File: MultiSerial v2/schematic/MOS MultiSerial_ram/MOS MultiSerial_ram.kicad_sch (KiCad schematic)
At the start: 36 parts, among them J10 ., J11 ., J12 Conn_01x01, J13 Conn_01x04, J14 Conn_01x02, J24 Conn_01x01, J6 Conn_01x04, J7 Conn_02x04_Odd_Even, J8 ., J9 Conn_01x01, U1 6551, U10 74AHC1G08, U2 74HC14, U3 65C52, U4 MC6850, U5 IS63WV1288DBLL-10xLI, U6 74LVC253, U7 74LVC595, U8 74AHC1G14

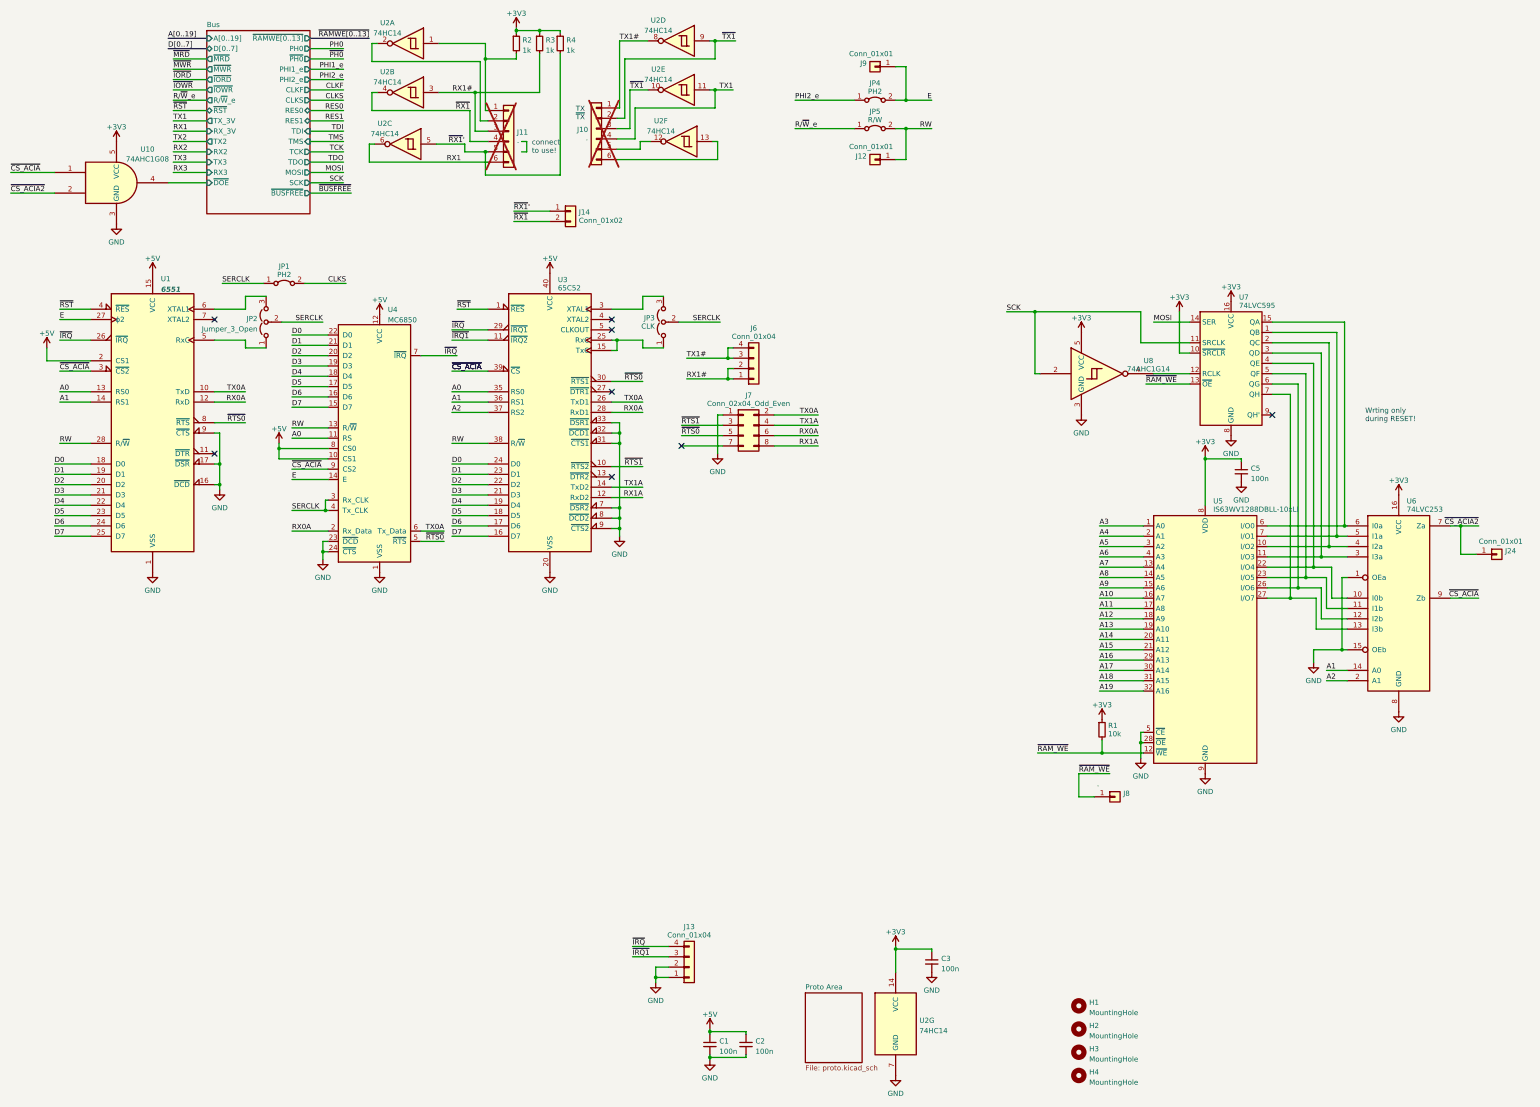
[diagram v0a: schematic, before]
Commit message: Documentation update
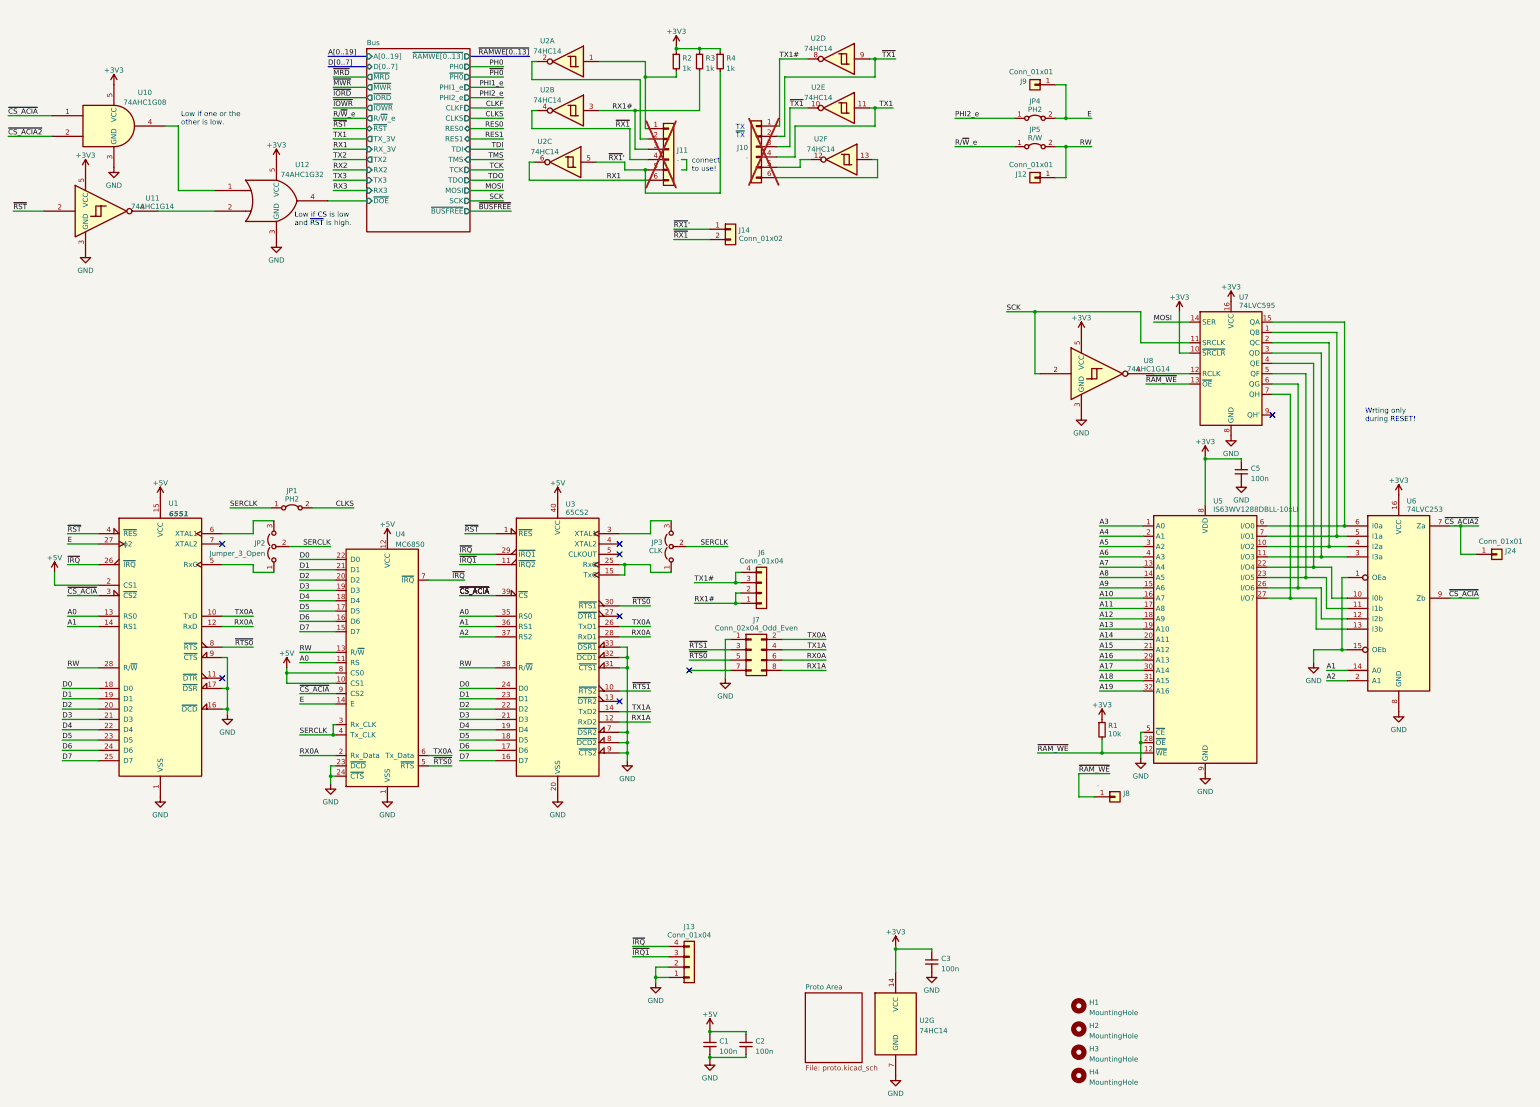
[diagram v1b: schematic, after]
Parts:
- added U11: 74AHC1G14, Package_TO_SOT_SMD:SOT-23-5, symbol 74xGxx:74AHC1G14
- added U12: 74AHC1G32, symbol 74xGxx:74AHC1G32
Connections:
- net +3V3: now also U11.5 (VCC), U12.5 (VCC)
- net Bus/~{DOE}: now also U12.4; no longer U10.4
- net GND: now also U11.3 (GND), U12.3 (GND)
- net ~{RST}: now also U11.2
- new net: U10.4, U12.1
- new net: U11.4, U12.2
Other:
- note added: "Low if CS is low and ~{RST} is high."
- note added: "Low if one or the other is low."
- moved on the sheet: J10, J11, J12, J14, J6, J7, J9, JP1, JP2, JP3, JP4, JP5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
